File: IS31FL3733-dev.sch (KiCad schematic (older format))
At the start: 22 parts, among them J1 Conn_01x11_Female, U1 IS31FL3733-QF

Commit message: Appearently buy parts is hard
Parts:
- C3, C5, C7: LCSC C307348 -> C80516; PN CL10B104KB8WPNC -> 0603B104K160CT
- R1, R2: LCSC C114668 -> C103303; PN RC0603FR-071K5L -> RTT031501FTP
- R3, R4, R5: LCSC C116674 -> C100703; PN AC0603FR-07100KL -> CR0603FA1003G
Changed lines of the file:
@@
 F 2 "Resistor_SMD:R_0603_1608Metric" V 1730 3450 50  0001 C CNN
 F 3 "~" H 1800 3450 50  0001 C CNN
-F 4 "C116674" H 1800 3450 50  0001 C CNN "LCSC"
-F 5 "AC0603FR-07100KL" H 1800 3450 50  0001 C CNN "PN"
+F 4 "C100703" H 1800 3450 50  0001 C CNN "LCSC"
+F 5 "CR0603FA1003G" H 1800 3450 50  0001 C CNN "PN"
 	1    1800 3450
 	-1   0    0    1
@@
 F 2 "Resistor_SMD:R_0603_1608Metric" V 2080 2650 50  0001 C CNN
 F 3 "~" H 2150 2650 50  0001 C CNN
-F 4 "C114668" H 2150 2650 50  0001 C CNN "LCSC"
-F 5 "RC0603FR-071K5L" H 2150 2650 50  0001 C CNN "PN"
+F 4 "C103303" H 2150 2650 50  0001 C CNN "LCSC"
+F 5 "RTT031501FTP" H 2150 2650 50  0001 C CNN "PN"
 	1    2150 2650
 	-1   0    0    1
@@
 F 2 "Resistor_SMD:R_0603_1608Metric" V 1830 2650 50  0001 C CNN
 F 3 "~" H 1900 2650 50  0001 C CNN
-F 4 "C114668" H 1900 2650 50  0001 C CNN "LCSC"
-F 5 "RC0603FR-071K5L" H 1900 2650 50  0001 C CNN "PN"
+F 4 "C103303" H 1900 2650 50  0001 C CNN "LCSC"
+F 5 "RTT031501FTP" H 1900 2650 50  0001 C CNN "PN"
 	1    1900 2650
 	-1   0    0    1
@@
 F 2 "Resistor_SMD:R_0603_1608Metric" V 2380 2650 50  0001 C CNN
 F 3 "~" H 2450 2650 50  0001 C CNN
-F 4 "C116674" H 2450 2650 50  0001 C CNN "LCSC"
-F 5 "AC0603FR-07100KL" H 2450 2650 50  0001 C CNN "PN"
+F 4 "C100703" H 2450 2650 50  0001 C CNN "LCSC"
+F 5 "CR0603FA1003G" H 2450 2650 50  0001 C CNN "PN"
 	1    2450 2650
 	-1   0    0    1
@@
 F 2 "Resistor_SMD:R_0603_1608Metric" V 1430 3450 50  0001 C CNN
 F 3 "~" H 1500 3450 50  0001 C CNN
-F 4 "C116674" H 1500 3450 50  0001 C CNN "LCSC"
-F 5 "AC0603FR-07100KL" H 1500 3450 50  0001 C CNN "PN"
+F 4 "C100703" H 1500 3450 50  0001 C CNN "LCSC"
+F 5 "CR0603FA1003G" H 1500 3450 50  0001 C CNN "PN"
 	1    1500 3450
 	-1   0    0    1
@@
 F 2 "Capacitor_SMD:C_0603_1608Metric" H 3488 2000 50  0001 C CNN
 F 3 "~" H 3450 2150 50  0001 C CNN
-F 4 "C307348" H 3450 2150 50  0001 C CNN "LCSC"
-F 5 "CL10B104KB8WPNC" H 3450 2150 50  0001 C CNN "PN"
+F 4 "C80516" H 3450 2150 50  0001 C CNN "LCSC"
+F 5 "0603B104K160CT" H 3450 2150 50  0001 C CNN "PN"
 	1    3450 2150
 	0    -1   -1   0
@@
 F 2 "Capacitor_SMD:C_0603_1608Metric" H 3888 2000 50  0001 C CNN
 F 3 "~" H 3850 2150 50  0001 C CNN
-F 4 "C307348" H 3850 2150 50  0001 C CNN "LCSC"
-F 5 "CL10B104KB8WPNC" H 3850 2150 50  0001 C CNN "PN"
+F 4 "C80516" H 3850 2150 50  0001 C CNN "LCSC"
+F 5 "0603B104K160CT" H 3850 2150 50  0001 C CNN "PN"
 	1    3850 2150
 	0    -1   -1   0
@@
 F 2 "Capacitor_SMD:C_0603_1608Metric" H 3688 1600 50  0001 C CNN
 F 3 "~" H 3650 1750 50  0001 C CNN
-F 4 "C307348" H 3650 1750 50  0001 C CNN "LCSC"
-F 5 "CL10B104KB8WPNC" H 3650 1750 50  0001 C CNN "PN"
+F 4 "C80516" H 3650 1750 50  0001 C CNN "LCSC"
+F 5 "0603B104K160CT" H 3650 1750 50  0001 C CNN "PN"
 	1    3650 1750
 	0    1    1    0

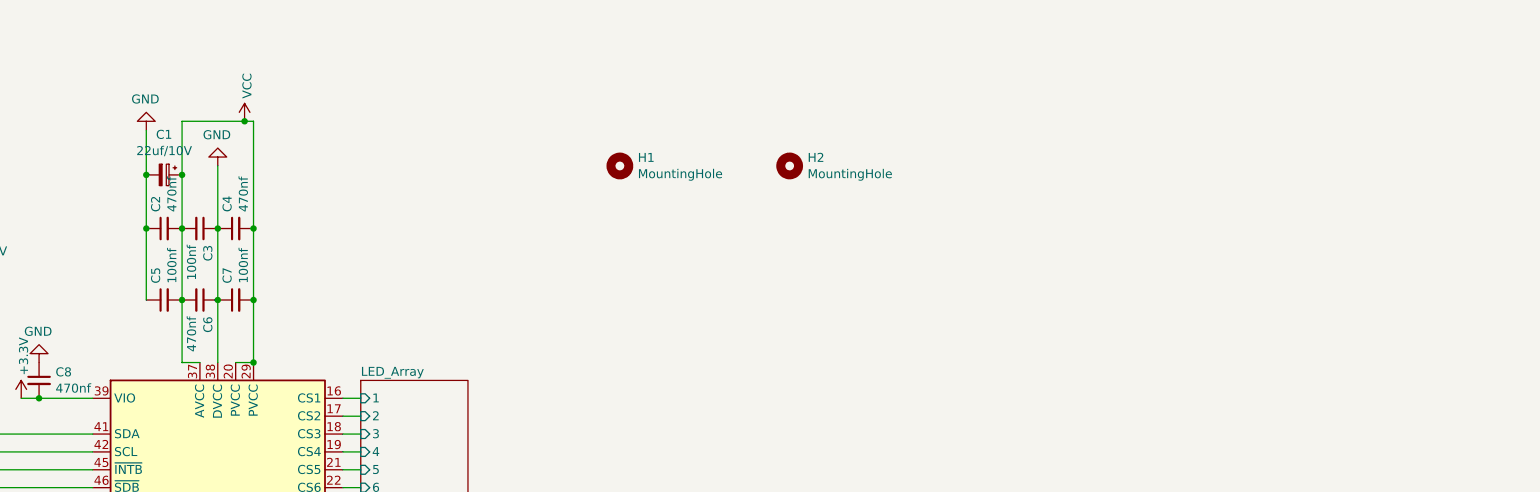
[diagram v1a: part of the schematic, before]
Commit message: fix problems with the board
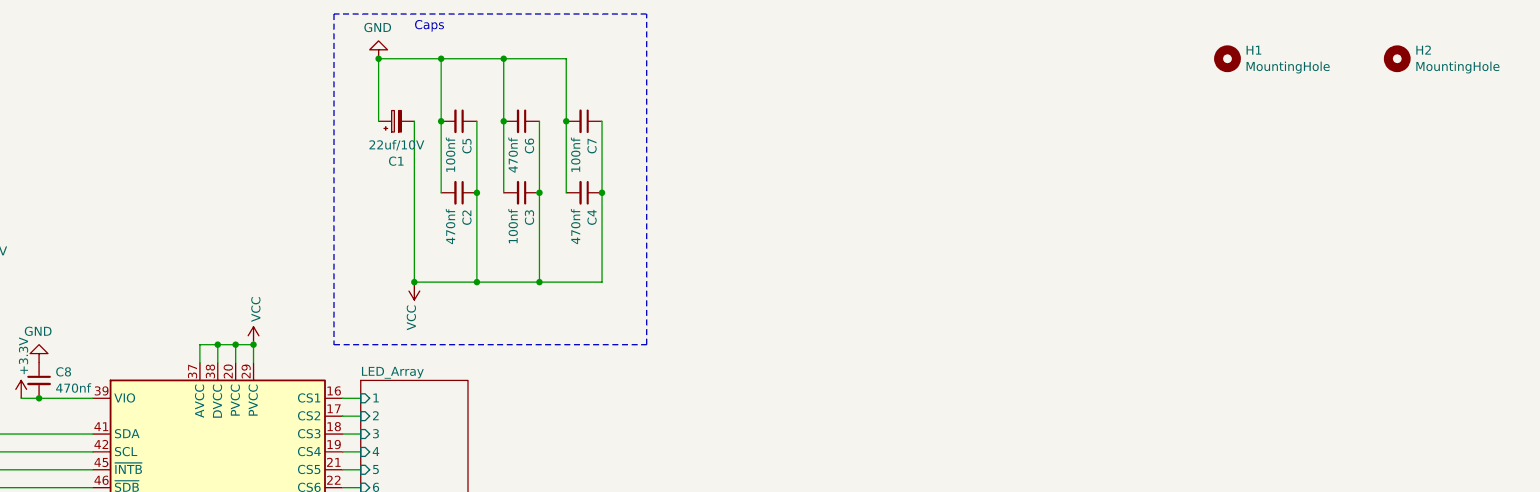
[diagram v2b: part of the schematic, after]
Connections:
- net GND: now also C1.1, C2.2, C3.2, C4.2, C5.2, C6.2, C7.2; no longer C1.2, C2.1, C3.1, C4.1, C5.1, C6.1, C7.1, U1.38 (DVCC)
- net VCC: now also C1.2, C2.1, C3.1, C4.1, C5.1, C6.1, C7.1, U1.38 (DVCC); no longer C1.1, C2.2, C3.2, C4.2, C5.2, C6.2, C7.2
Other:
- note added: "Caps"
- moved on the sheet: C1, C2, C3, C4, C5, C6, C7, H1, H2
